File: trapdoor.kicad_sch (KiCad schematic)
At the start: 2 parts, among them P9 TRAPDOOR

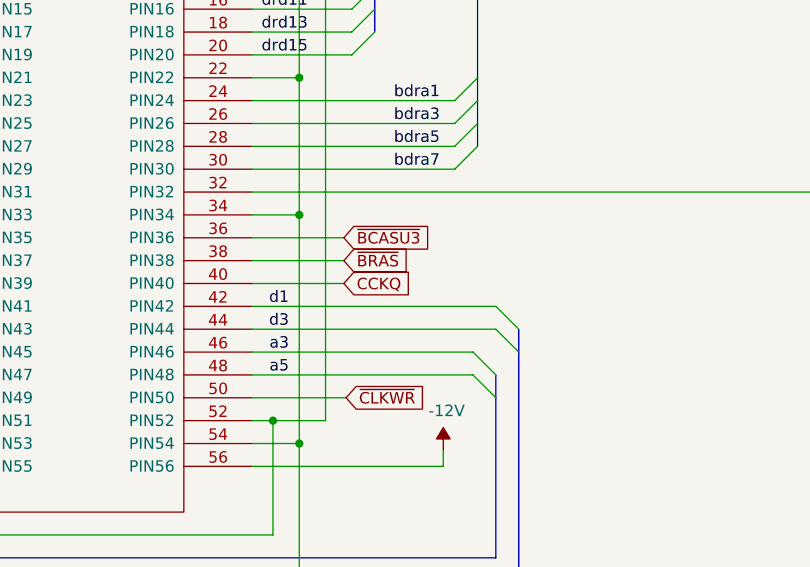
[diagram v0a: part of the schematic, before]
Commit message: removed JP2
some more small fixes
schematic is now more or less done I think
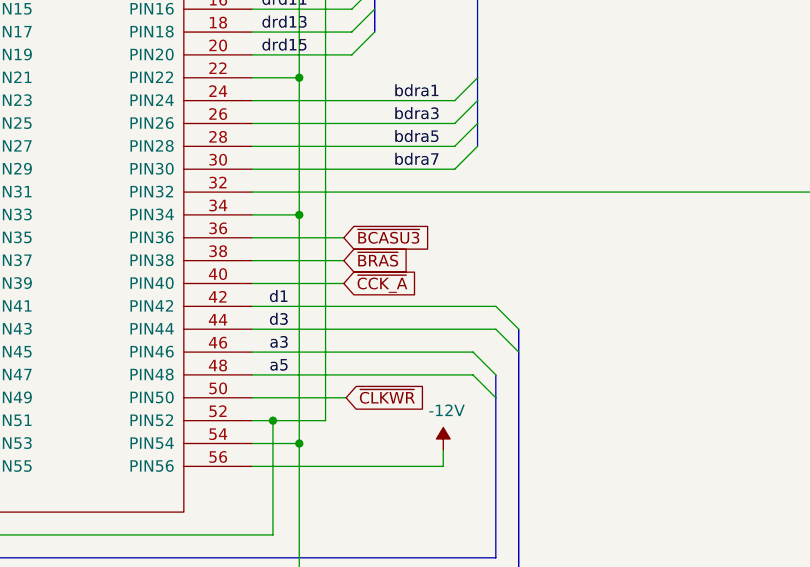
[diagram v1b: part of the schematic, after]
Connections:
- net CCKQ renamed ~{CCK_A}
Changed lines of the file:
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@@
 		)
 	)
-	(global_label "CCKQ"
+	(global_label "~{CCK_A}"
 		(shape input)
 		(at 185.42 109.22 0)
